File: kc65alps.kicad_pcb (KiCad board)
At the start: 2 copper layers, 160 parts, among them J1 Conn_01x04, J2 AVR-ISP-6, U1 ATmega32U4-AU, Y1 16MHz

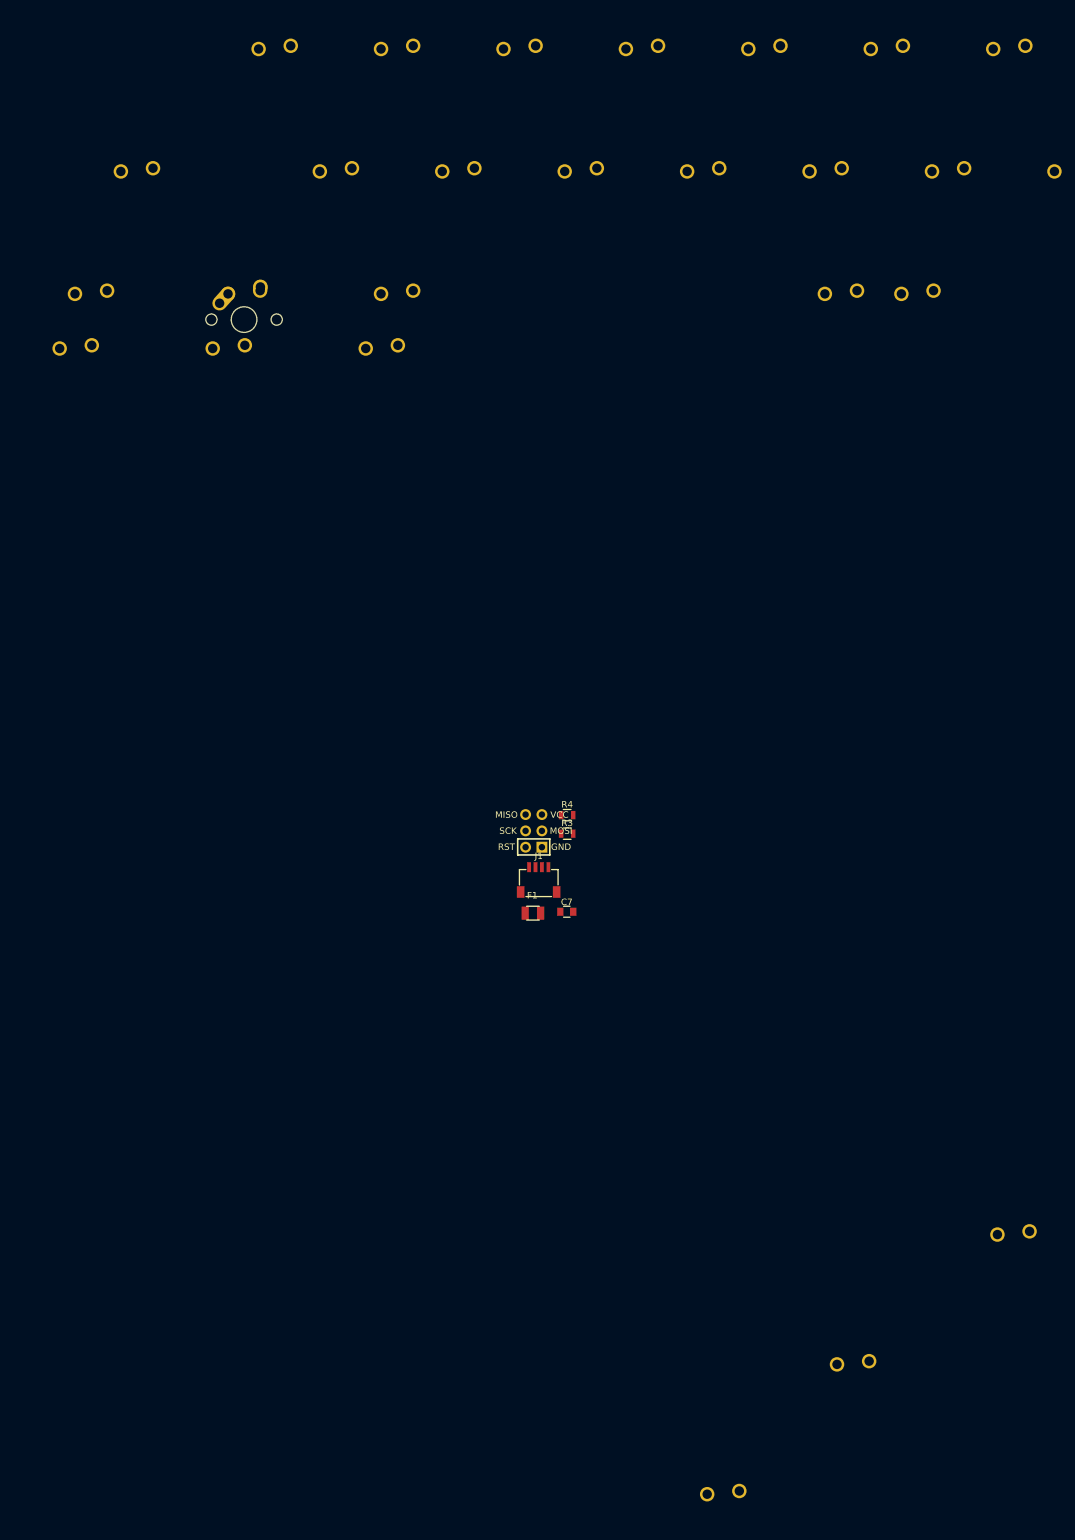
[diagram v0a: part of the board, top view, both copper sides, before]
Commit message: PCB update
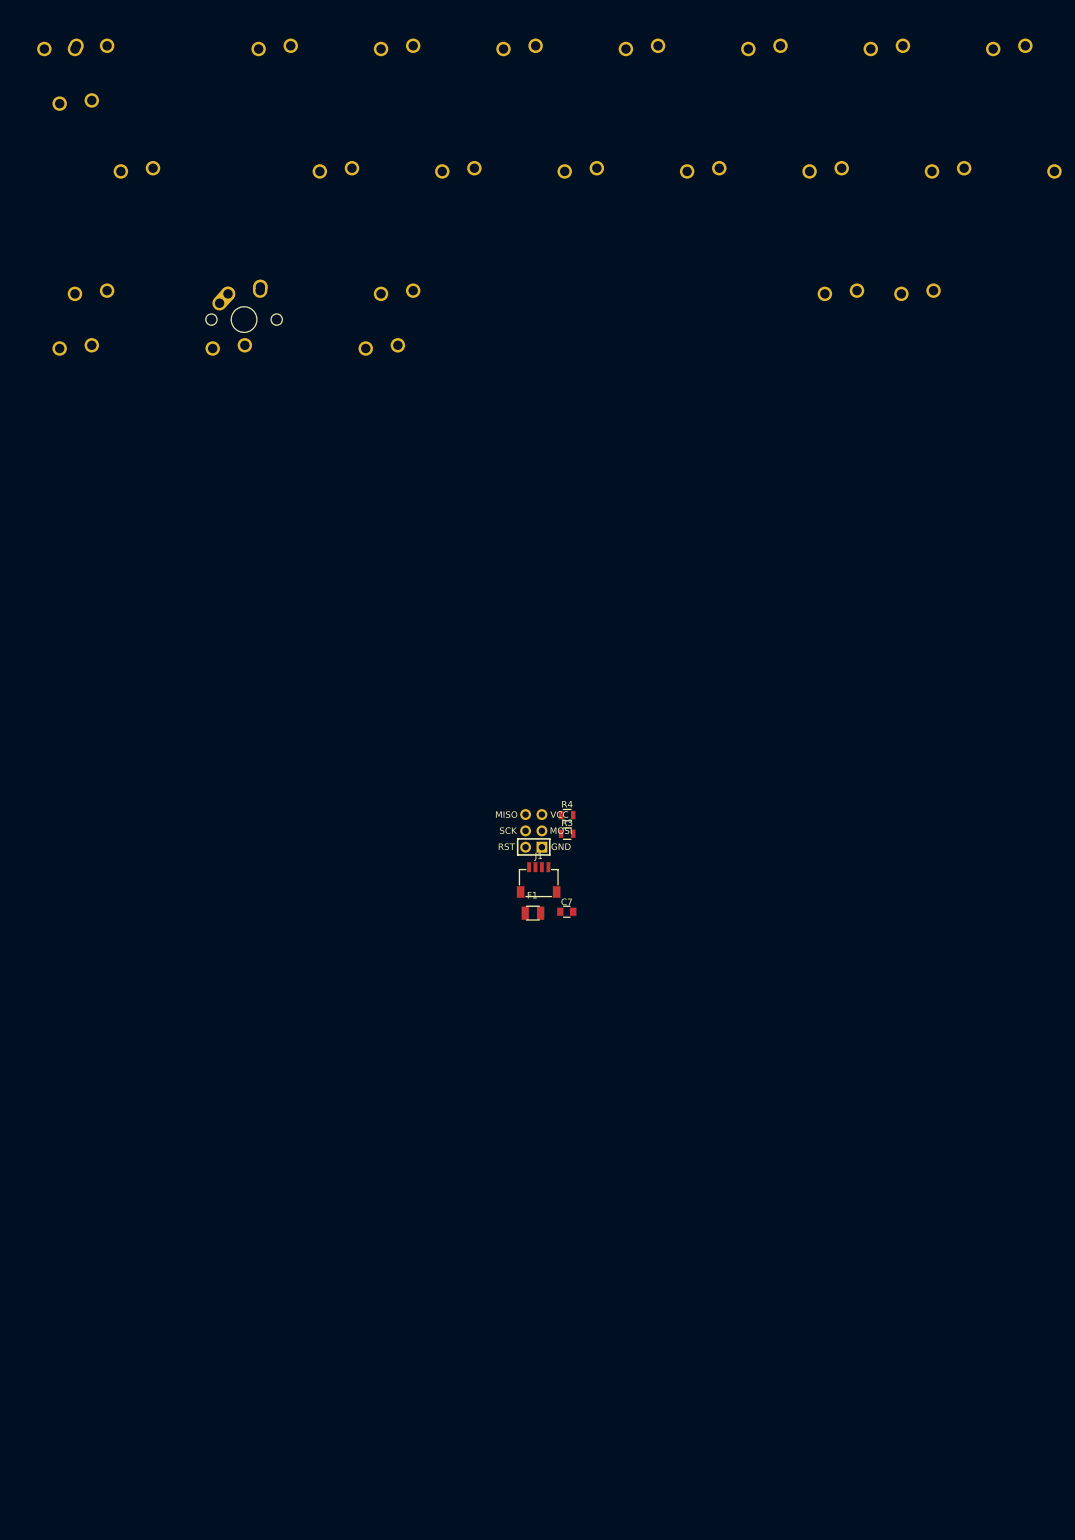
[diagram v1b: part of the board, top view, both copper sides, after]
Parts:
- moved MX-Caps3 246.4 mm to (31.0, 127.0), turned to 180 degrees
- moved MX-Caps2 239.0 mm to (28.6, 127.0)
- moved MX-Caps1 233.7 mm to (33.3, 127.0)
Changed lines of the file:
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@@
     (solder_mask_min_width 0.25)
     (aux_axis_origin 0 0)
-    (visible_elements FFFFFF7F)
+    (visible_elements 7FFFF7FF)
     (pcbplotparams
       (layerselection 0x010fc_ffffffff)
@@
   )
   (module Alps_Only:ALPS-1U (layer F.Cu)
-    (at 131.7075 351.865)
+    (at 30.95625 127 180)
     (fp_text reference MX-Caps3 (at 0 3.175) (layer Dwgs.User)
       (effects (font (size 1 1) (thickness 0.15)))
@@
     (fp_line (start 7 -7) (end 7 -5) (layer Dwgs.User) (width 0.15))
     (fp_line (start 5 -7) (end 7 -7) (layer Dwgs.User) (width 0.15))
-    (pad 1 thru_hole circle (at -2.5 -4) (size 2.25 2.25) (drill 1.47) (layers *.Cu B.Mask)
+    (pad 1 thru_hole circle (at -2.5 -4 180) (size 2.25 2.25) (drill 1.47) (layers *.Cu B.Mask)
       (net 40 "Net-(D32-Pad2)"))
-    (pad 2 thru_hole circle (at 2.5 -4.5) (size 2.25 2.25) (drill 1.47) (layers *.Cu B.Mask)
+    (pad 2 thru_hole circle (at 2.5 -4.5 180) (size 2.25 2.25) (drill 1.47) (layers *.Cu B.Mask)
       (net 100 COL0))
   )
   (module Alps_Only:ALPS-1U (layer F.Cu)
-    (at 151.9075 331.665)
+    (at 28.575 127)
     (fp_text reference MX-Caps2 (at 0 3.175) (layer Dwgs.User)
       (effects (font (size 1 1) (thickness 0.15)))
@@
   )
   (module Alps_Only:ALPS-1U (layer F.Cu)
-    (at 176.8675 311.465)
+    (at 33.3375 127)
     (fp_text reference MX-Caps1 (at 0 3.175) (layer Dwgs.User)
       (effects (font (size 1 1) (thickness 0.15)))

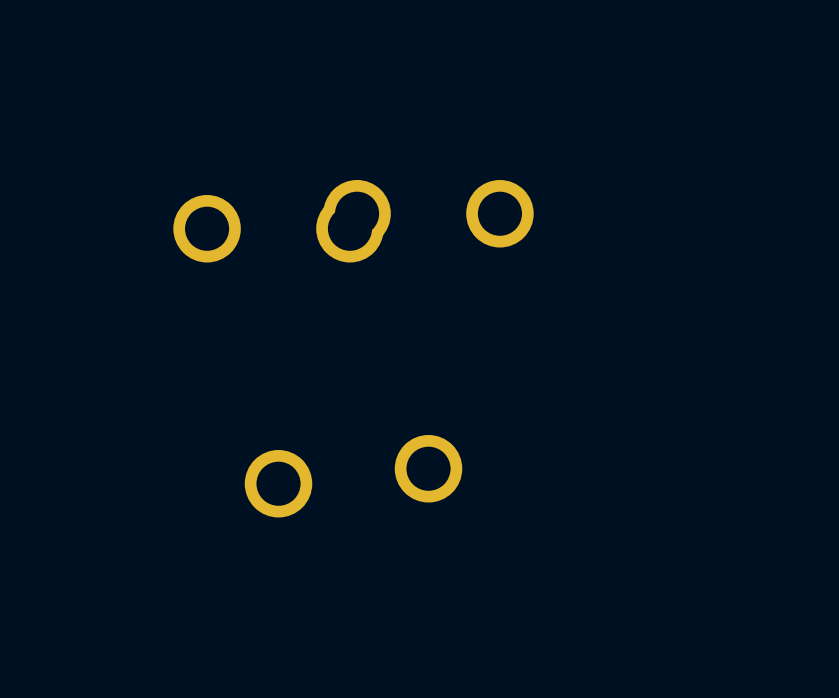
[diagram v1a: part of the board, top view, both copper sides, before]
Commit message: PCB update
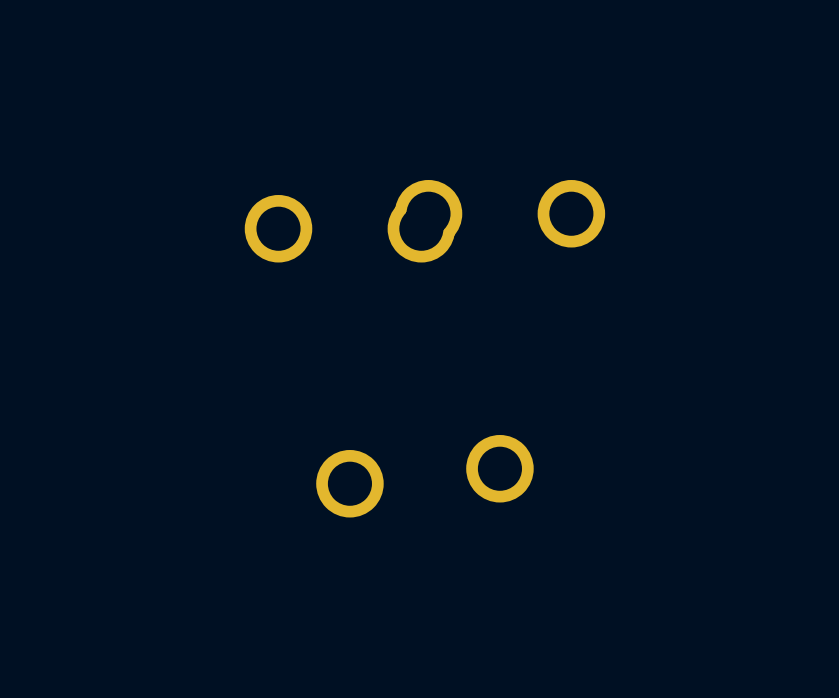
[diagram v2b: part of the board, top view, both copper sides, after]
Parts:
- moved MX-Caps1 2.38 mm to (35.7, 127.0)
- moved MX-Caps2 2.38 mm to (31.0, 127.0)
- moved MX-Caps3 2.38 mm to (33.3, 127.0)
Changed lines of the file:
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@@
   )
   (module Alps_Only:ALPS-1U (layer F.Cu)
-    (at 30.95625 127 180)
+    (at 33.3375 127 180)
     (fp_text reference MX-Caps3 (at 0 3.175) (layer Dwgs.User)
       (effects (font (size 1 1) (thickness 0.15)))
@@
   )
   (module Alps_Only:ALPS-1U (layer F.Cu)
-    (at 28.575 127)
+    (at 30.95625 127)
     (fp_text reference MX-Caps2 (at 0 3.175) (layer Dwgs.User)
       (effects (font (size 1 1) (thickness 0.15)))
@@
   )
   (module Alps_Only:ALPS-1U (layer F.Cu)
-    (at 33.3375 127)
+    (at 35.71875 127)
     (fp_text reference MX-Caps1 (at 0 3.175) (layer Dwgs.User)
       (effects (font (size 1 1) (thickness 0.15)))
